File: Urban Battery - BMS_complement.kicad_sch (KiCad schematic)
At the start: 41 parts, among them J1 BMS IO, J10 E-Stop, J11 Contactor Connector, J12 Thermistor, J13 Thermistor, J14 Thermistor, J2 OLED Header, J3 CAN, J4 CAN, J5 Charge Connector, J6 Battery Connector, J7 E-Stop, J8 E-Stop, J9 E-Stop, K1 Charge_Relay, K2 Contactor_Relay, SW1 SW_SPST, SW2 SW_DPDT_x2, SW3 CAN_TERM, U1 MCP2515-I/SO, U2 MCP2561/2, U3 LM2575HVS-12/NOPB, Y1 8MHz

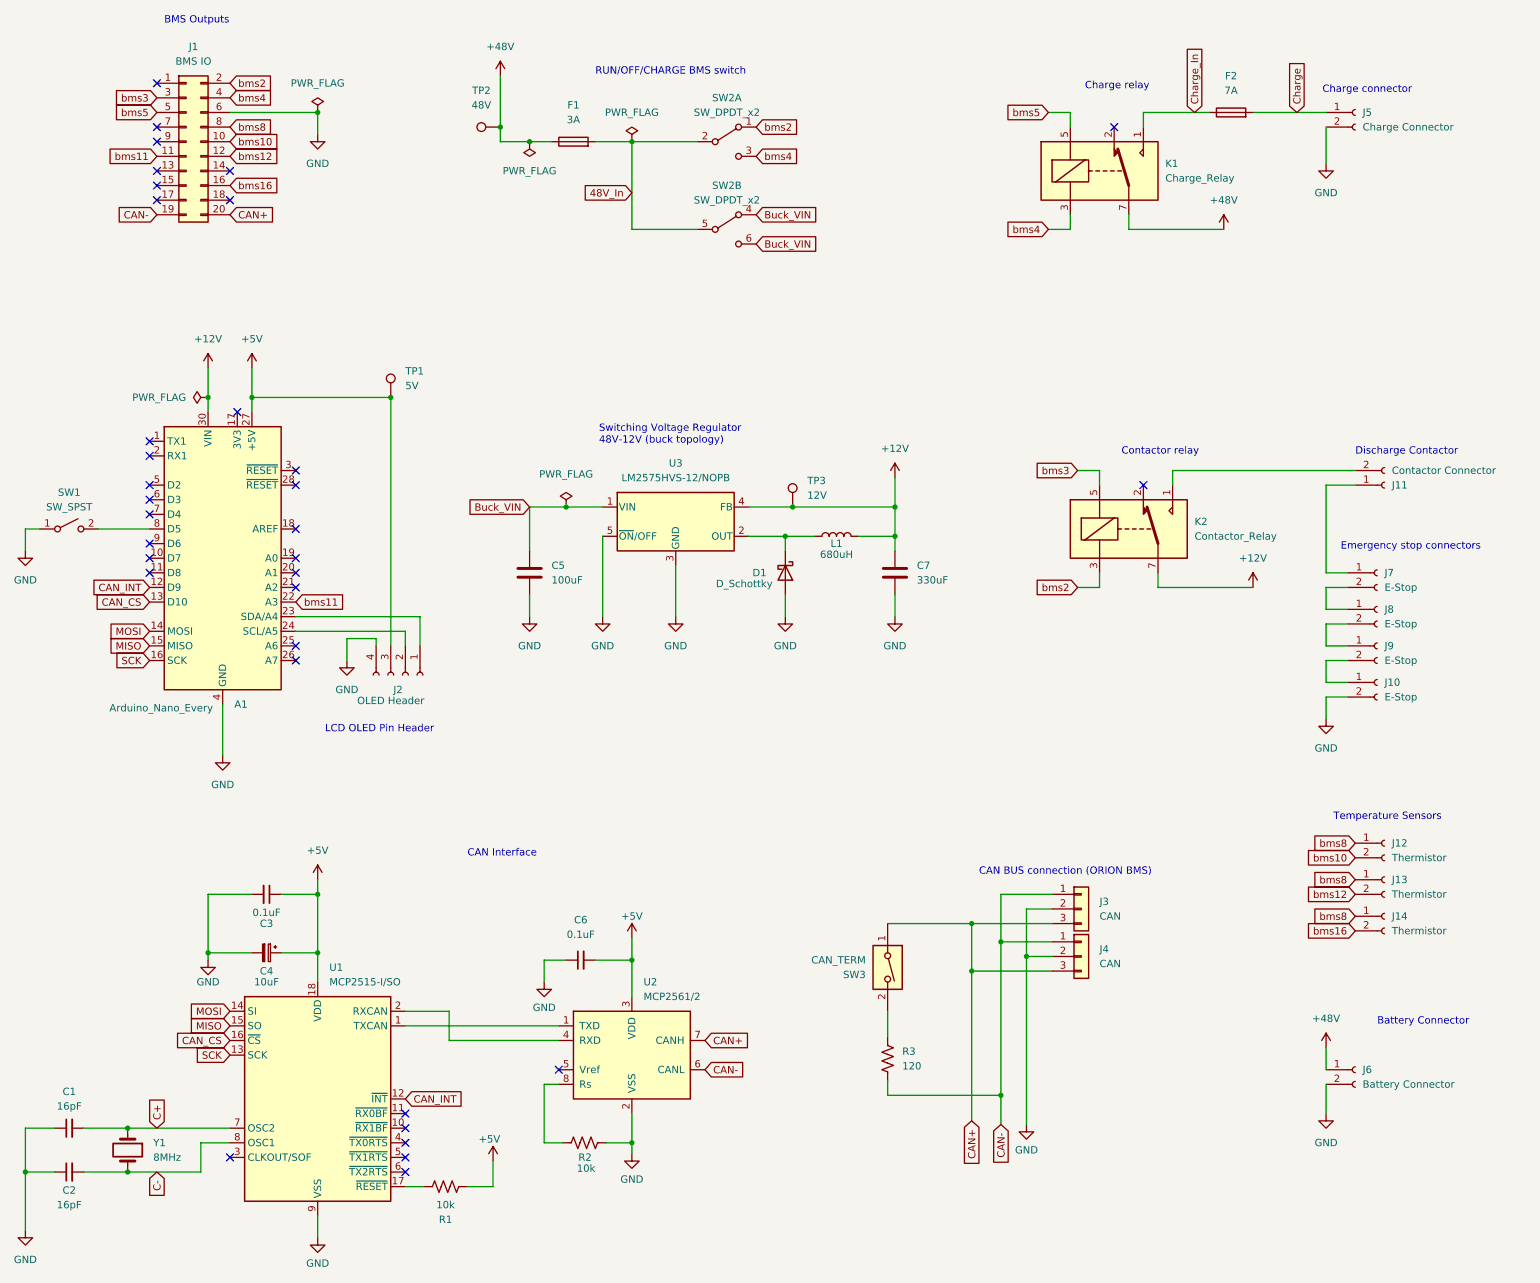
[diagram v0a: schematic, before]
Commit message: only pushing to verify no accidental changes were made before more people work on this again
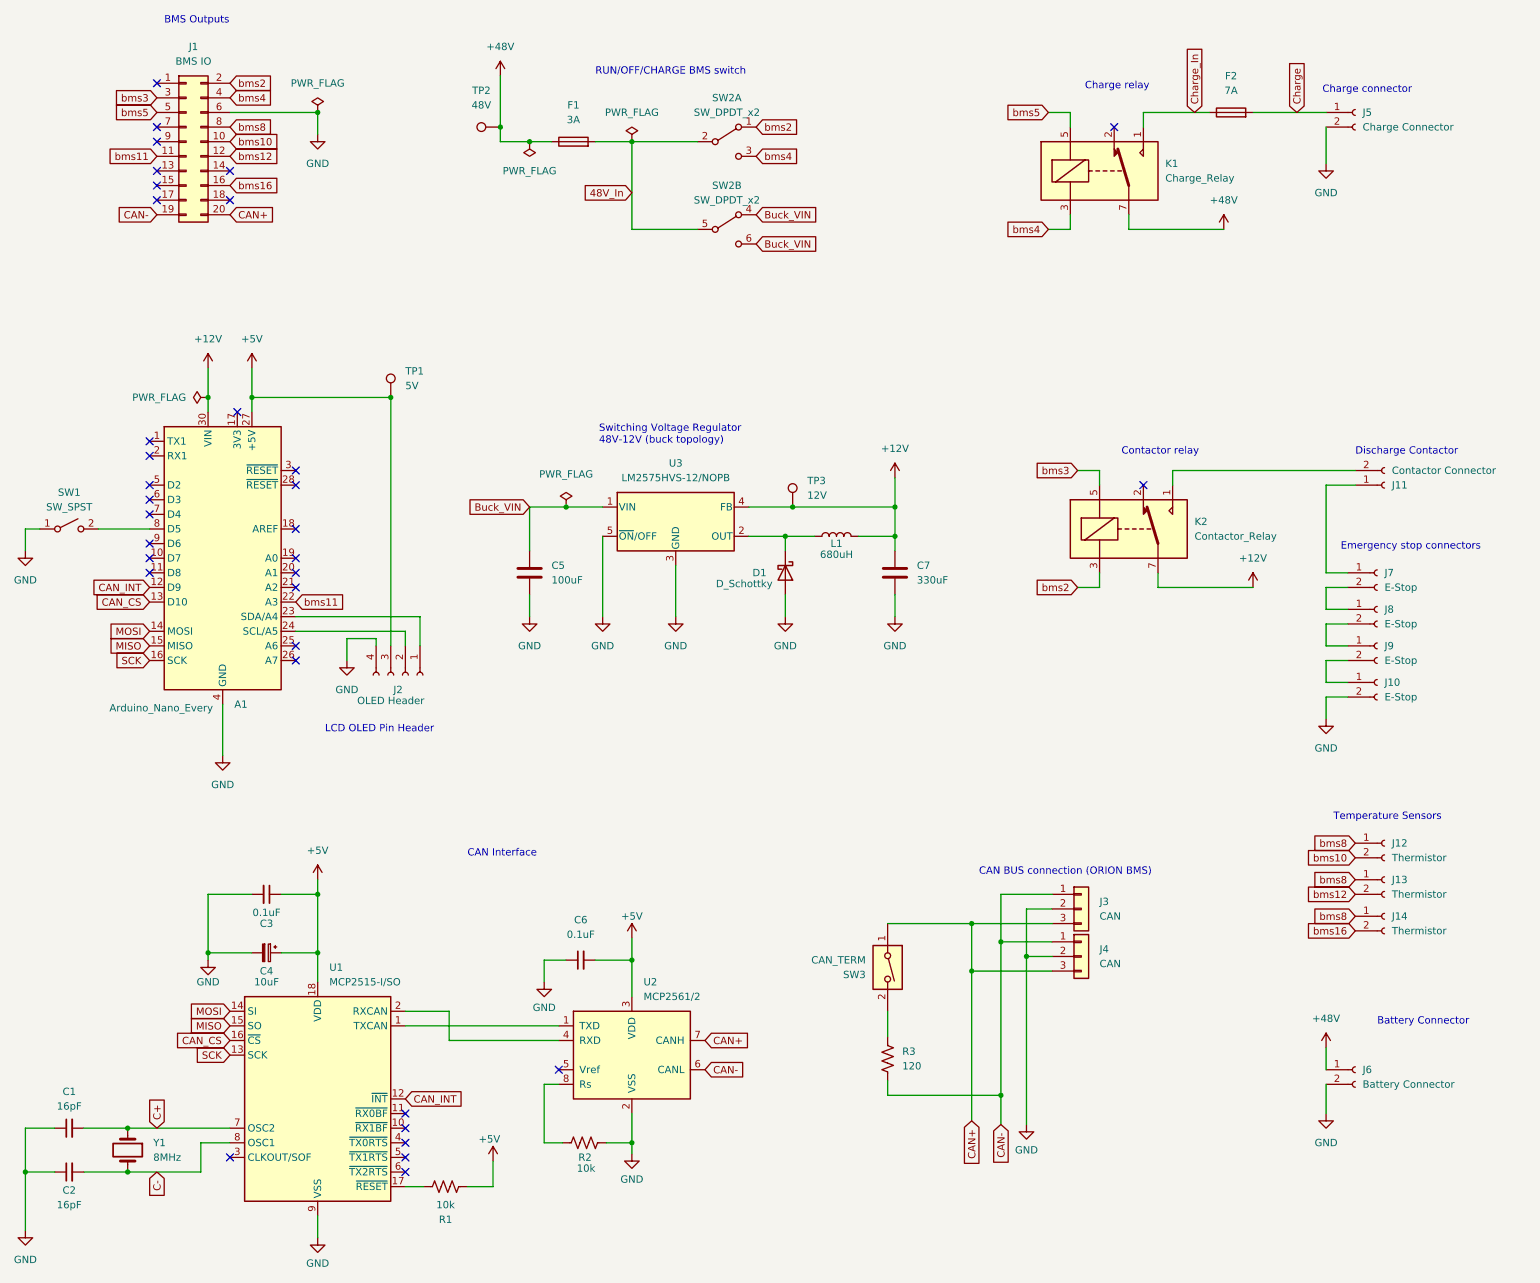
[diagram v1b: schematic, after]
